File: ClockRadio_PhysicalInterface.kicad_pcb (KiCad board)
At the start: 2 copper layers, 155.6 x 31.8 mm, 77 parts, among them J1 Interface_tether, SW1 SW_Push, SW2 5WAY_SW, U1 TC1262-33, U2 PCA9685PW

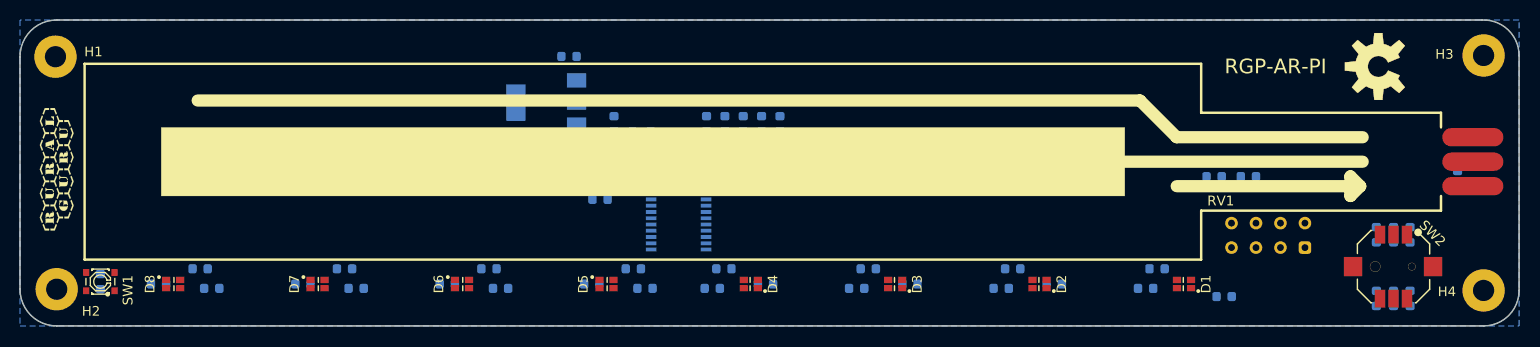
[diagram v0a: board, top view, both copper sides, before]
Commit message: Schematic and layout complete
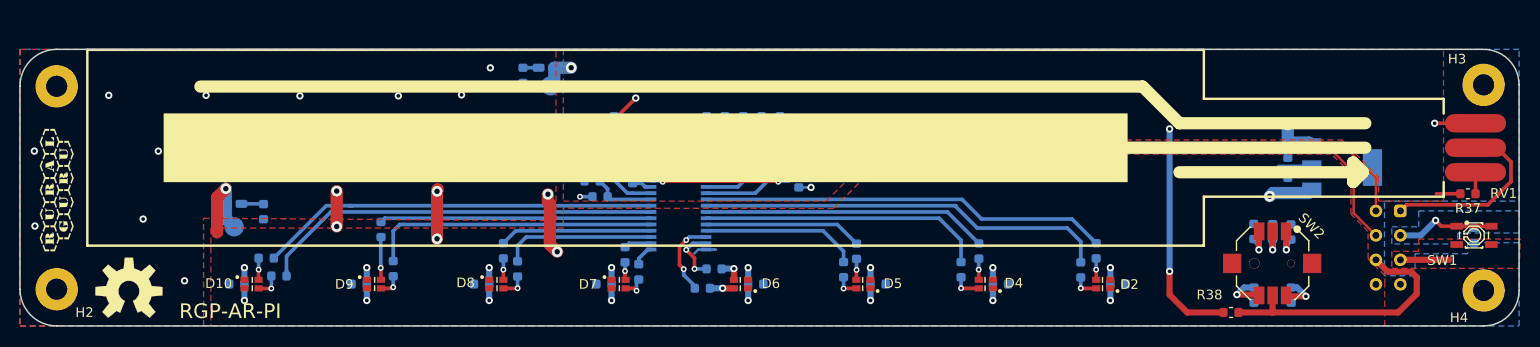
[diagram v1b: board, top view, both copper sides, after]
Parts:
- added D10: BL-OR, ERW_LED:Double_LED_0603_1608Metric_Castellated, F.Cu at (49.4, 52.8)
- added D9: BL-OR, ERW_LED:Double_LED_0603_1608Metric_Castellated, F.Cu at (62.1, 52.8)
- added R42: 3.3k, Resistor_SMD:R_0603_1608Metric, B.Cu at (157.3, 47.4)
- added R43: 10k, Resistor_SMD:R_0603_1608Metric, B.Cu at (155.4, 47.4)
- added TP1: TestPoint, TestPoint:TestPoint_Pad_D2.0mm, B.Cu at (47.6, 46.9)
- added TP2: TestPoint, TestPoint:TestPoint_Pad_D2.0mm, B.Cu at (80.5, 32.2)
- D1, D3: value BL-OR -> GRN; footprint ERW_LED:Double_LED_0603_1608Metric_Castellated -> LED_SMD:LED_0603_1608Metric_Castellated; moved to B.Cu
- R1: value 150Ω -> 120Ω
- R10: value 150Ω -> 100Ω
- R11, R19, R25, R35: value 1k -> 200Ω
- R12, R24, R34: value 1k -> 150Ω
- R17, R21, R31: value 200Ω -> 1k
- R2: value 200Ω -> 150Ω
- R20, R30: value 150Ω -> 1k
- R3, R6: value 150Ω -> 200Ω
- R36: value 10k -> 1k
- R37: value 330Ω -> 1k; moved to F.Cu
- R38: value 680Ω -> 10k; moved to F.Cu
- R39: value 1.5k -> 330Ω
- R4: value 10k -> 150Ω
- R40: value 3.3k -> 680Ω
- R41: value 10k -> 1.5k
- R5: value 200Ω -> 10k
- R7: value 0Ω -> 150Ω
- R8: value 100Ω -> 200Ω
- R9: value 200Ω -> 0Ω
- moved SW1 142.6 mm to (176.3, 47.8), turned to 0 degrees
- moved G1 131.7 mm to (36.7, 53.5), turned to 0 degrees
- moved G2 131.7 mm to (36.7, 53.5), turned to 180 degrees
- moved G3 131.7 mm to (36.7, 53.5), turned to 0 degrees
- moved G4 131.7 mm to (36.7, 53.5), turned to 180 degrees
- moved R35 123.9 mm to (51.0, 50.1), turned to 0 degrees
- moved U1 82.9 mm to (162.6, 40.7), turned to 0 degrees
- moved C4 75.8 mm to (157.0, 42.6), turned to 90 degrees
- moved C6 74.6 mm to (157.0, 38.9), turned to 270 degrees
- moved D1 69.9 mm to (80.0, 30.4), turned to 0 degrees
- moved D3 69.2 mm to (47.6, 44.5), turned to 180 degrees
- moved R1 68.8 mm to (77.6, 31.1), turned to 270 degrees
- moved R18 56.4 mm to (96.6, 37.7), turned to 90 degrees
- moved R19 52.8 mm to (97.4, 51.2)
- moved R5 42.7 mm to (85.6, 43.7), turned to 0 degrees
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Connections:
- D1 pad 1: V6P0 -> /V3P3_LED
- D1 pad 2: V6P0 -> V3P3
- D2 pad 3: /BL2 -> /BL1
- D2 pad 4: /OR2 -> /OR1
- D3 pad 1: V6P0 -> /V6P0_LED
- D4 pad 3: /BL4 -> /BL2
- D4 pad 4: /OR4 -> /OR2
- D5 pad 3: /BL5 -> /BL3
- D5 pad 4: /OR5 -> /OR3
- D6 pad 3: /BL6 -> /BL4
- D6 pad 4: /OR6 -> /OR4
- D7 pad 3: /BL7 -> /BL5
- D7 pad 4: /OR7 -> /OR5
- D8 pad 3: /BL8 -> /BL6
- D8 pad 4: /OR8 -> /OR6
- J1 pad 1: PI_5way -> PI_pot
- J1 pad 2: SYTEM_POWER -> I2C_SCL
- J1 pad 3: PI_pot -> SYTEM_POWER
- J1 pad 4: STBY -> I2C_SDA
- J1 pad 5: I2C_SDA -> STBY
- J1 pad 6: I2C_SCL -> PI_5way
- R1 pad 1: /OR1 -> /V3P3_LED
- R1 pad 2: /LED1a -> GND
- R10 pad 1: /BL4 -> /Output_Enable
- R10 pad 2: /LED4a -> GND
- R11 pad 1: V3P3 -> /BL3
- R11 pad 2: /A5_SEL -> /LED3b
- R12 pad 1: V3P3 -> /BL4
- R12 pad 2: /A4_SEL -> /LED4a
- R13 pad 2: /A3_SEL -> /A5_SEL
- R14 pad 2: /A2_SEL -> /A4_SEL
- R15 pad 2: /A1_SEL -> /A3_SEL
- R16 pad 2: /A0_SEL -> /A2_SEL
- R17 pad 1: /OR4 -> V3P3
- R17 pad 2: /LED4b -> /A1_SEL
- R18 pad 1: V6P0 -> V3P3
- R18 pad 2: I2C_SCL -> /A0_SEL
- R19 pad 1: V6P0 -> /OR4
- R19 pad 2: I2C_SDA -> /LED4b
- R2 pad 1: /BL1 -> /OR1
- R2 pad 2: /LED1b -> /LED1a
- R20 pad 1: /OR5 -> V3P3
- R20 pad 2: /LED5a -> I2C_SDA
- R21 pad 1: /BL5 -> V3P3
- R21 pad 2: /LED5b -> I2C_SCL
- R22 pad 1: /OR6 -> /OR5
- R22 pad 2: /LED6a -> /LED5a
- R23 pad 1: /BL6 -> /BL5
- R23 pad 2: /LED6b -> /LED5b
- R24 pad 1: /A5_SEL -> /OR6
- R24 pad 2: GND -> /LED6a
- R25 pad 1: /A4_SEL -> /BL6
- R25 pad 2: GND -> /LED6b
- R26 pad 1: /A3_SEL -> /A5_SEL
- R27 pad 1: /A2_SEL -> /A4_SEL
- R28 pad 1: /A1_SEL -> /A3_SEL
- R29 pad 1: /A0_SEL -> /A2_SEL
- R3 pad 1: /OR2 -> /BL1
- R3 pad 2: /LED2a -> /LED1b
- R30 pad 1: /OR7 -> /A1_SEL
- R30 pad 2: /LED7a -> GND
- R31 pad 1: /BL7 -> /A0_SEL
- R31 pad 2: /LED7b -> GND
- R32 pad 1: /OR8 -> /OR7
- R32 pad 2: /LED8a -> /LED7a
- R33 pad 1: /BL8 -> /BL7
- R33 pad 2: /LED8b -> /LED7b
- R34 pad 1: SYTEM_POWER -> /OR8
- R34 pad 2: GND -> /LED8a
- R35 pad 1: V3P3 -> /BL8
- R35 pad 2: Net-(R35-Pad2) -> /LED8b
- R36 pad 1: V3P3 -> SYTEM_POWER
- R36 pad 2: PI_5way -> GND
- R37 pad 1: Net-(R37-Pad1) -> V3P3
- R37 pad 2: GND -> /pot_pullup
- R38 pad 1: Net-(R38-Pad1) -> V3P3
- R38 pad 2: GND -> PI_5way
- R39 pad 1: Net-(R39-Pad1) -> /SW_Right
- R4 pad 1: V3P3 -> /OR2
- R4 pad 2: /Output_Enable -> /LED2a
- R40 pad 1: Net-(R40-Pad1) -> /SW_Left
- R41 pad 1: Net-(R41-Pad1) -> /SW_Down
- R5 pad 1: /BL2 -> V3P3
- R5 pad 2: /LED2b -> /Output_Enable
- R6 pad 1: /OR3 -> /BL2
- R6 pad 2: /LED3a -> /LED2b
- R7 pad 1: /CLK_EXT -> /OR3
- R7 pad 2: GND -> /LED3a
- R8 pad 1: /Output_Enable -> /V6P0_LED
- R9 pad 1: /BL3 -> /CLK_EXT
- R9 pad 2: /LED3b -> GND
- RV1 pad 1: Net-(R35-Pad2) -> /pot_pullup
- SW2 pad 1: Net-(R40-Pad1) -> /SW_UP
- SW2 pad 2: Net-(R41-Pad1) -> /SW_Center
- SW2 pad 3: Net-(R38-Pad1) -> /SW_Left
- SW2 pad 4: Net-(R37-Pad1) -> /SW_Right
- SW2 pad 6: Net-(R39-Pad1) -> /SW_Down
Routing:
- net I2C_SDA: track 0.00 -> 82.3 mm, vias 0 -> 3
- net I2C_SCL: track 0.00 -> 81.9 mm, vias 0 -> 3
- net V3P3: track 0.00 -> 49.6 mm, vias 0 -> 14
- net /LED1b: track 0.00 -> 42.7 mm
- net /LED1a: track 0.00 -> 42.4 mm
- net /LED8a: track 0.00 -> 41.8 mm
- net /LED8b: track 0.00 -> 41.7 mm
- net V6P0: track 0.00 -> 41.1 mm, vias 0 -> 18
- net GND: track 0.00 -> 34.9 mm, vias 0 -> 24
- net /LED7a: track 0.00 -> 30.2 mm
- net /LED2b: track 0.00 -> 29.7 mm
- net /LED2a: track 0.00 -> 29.7 mm
- net /LED7b: track 0.00 -> 28.2 mm
- net PI_5way: track 0.00 -> 27.8 mm
- net PI_pot: track 0.00 -> 19.1 mm
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- added copper zone on F.Cu, net GND
- added copper zone on F.Cu, net STBY
- added copper zone on B.Cu, net SYTEM_POWER
- added copper zone on F.Cu, net V3P3
- added copper zone on F.Cu, net V6P0
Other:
- board size 155.6 x 31.8 mm -> 155.6 x 28.7 mm
- net class Default: clearance 0.2 -> 0.1524; trace_width 0.25 -> 0.1524; via_dia 0.8 -> 0.762; via_drill 0.4 -> 0.381
- net class LED_20mA added: clearance 0.2032, trace_width 0.254, via_dia 0.762, via_drill 0.381
- net class PWR added: clearance 0.254, trace_width 0.254, via_dia 0.762, via_drill 0.381
- rule trace_clearance: 0.2 -> 0.1524
- rule trace_min: 0.2 -> 0.127
- rule via_min_drill: 0.3 -> 0.3048
- rule via_min_size: 0.4 -> 0.6096
